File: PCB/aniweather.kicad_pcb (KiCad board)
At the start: 2 copper layers, 55 x 75 mm, 32 parts, among them SW1 SW_DIP_x01, SW2 SW_Push, SW3 SW_Push, U5 TPS63001

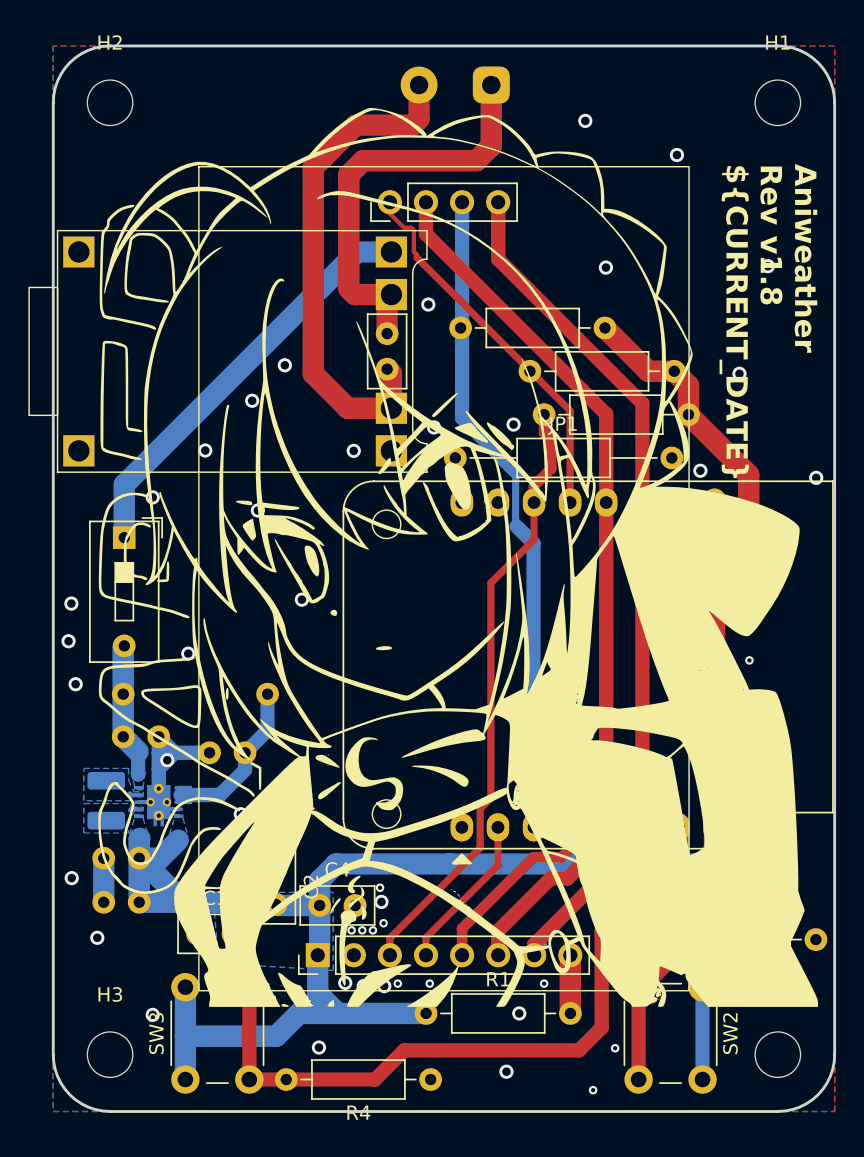
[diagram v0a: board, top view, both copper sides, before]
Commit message: PCB revision
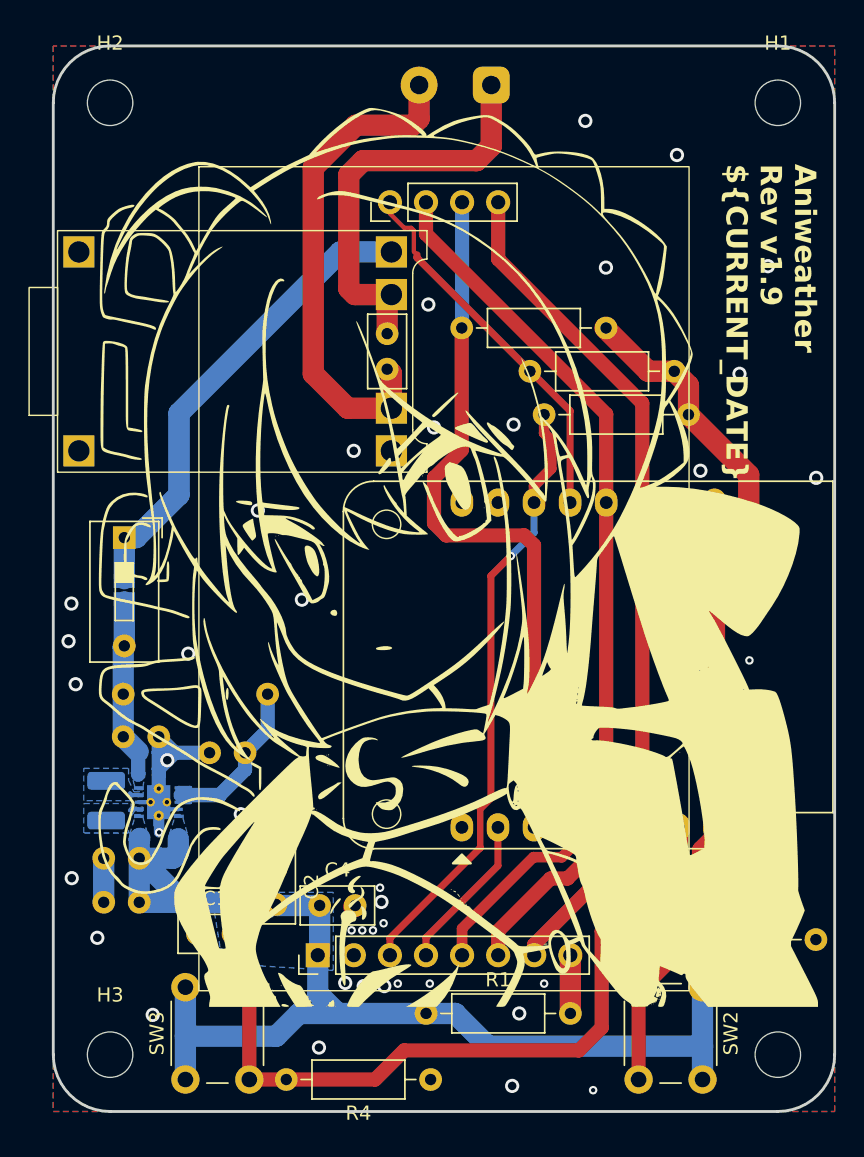
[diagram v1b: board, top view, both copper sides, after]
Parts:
- JP1: value Jumper_2_Bridged -> Jumper_2_Open; footprint Resistor_THT:R_Axial_DIN0207_L6.3mm_D2.5mm_P15.24mm_Horizontal -> Jumper:SolderJumper-2_P1.3mm_Open_Pad1.0x1.5mm; moved to B.Cu
- moved JP1 25.1 mm to (117.7, 101.7), turned to 90 degrees
- moved R7 0.08 mm to (141.4, 83.3)
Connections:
- C6 pad 1: Net-(U5-VIN) -> Net-(JP1-A)
- JP1 pad 1: GND -> Net-(JP1-A)
- JP1 pad 2: GND -> Net-(JP1-B)
- R2 pad 2: Net-(U5-VIN) -> Net-(JP1-A)
- SW1 pad 1: Net-(U3-OUT+) -> Net-(JP1-B)
- SW1 pad 2: Net-(U5-VIN) -> Net-(JP1-A)
- U3 pad 2: Net-(U3-OUT+) -> Net-(JP1-B)
- U5 pad 5: Net-(U5-VIN) -> Net-(JP1-A)
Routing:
- net Net-(JP1-B): track 0.00 -> 33.4 mm
- net Net-(U3-OUT+): track 29.3 -> 0.00 mm
- net Net-(JP1-A): track 0.00 -> 12.6 mm
- net Net-(U5-VIN): track 9.54 -> 0.00 mm
- net +3.3V: track 146.4 -> 138.6 mm
- net MISO: track 46.1 -> 51.0 mm
- net GND: track 17.0 -> 18.2 mm, vias 53 -> 49
- net CS_LCD: vias 0 -> 1
- added copper zone on B.Cu, net Net-(JP1-A)
- removed copper zone on B.Cu, net Net-(U5-VIN)
